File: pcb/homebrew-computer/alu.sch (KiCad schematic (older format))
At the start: 4 parts, among them U4 XC9572XL-10VQG44C

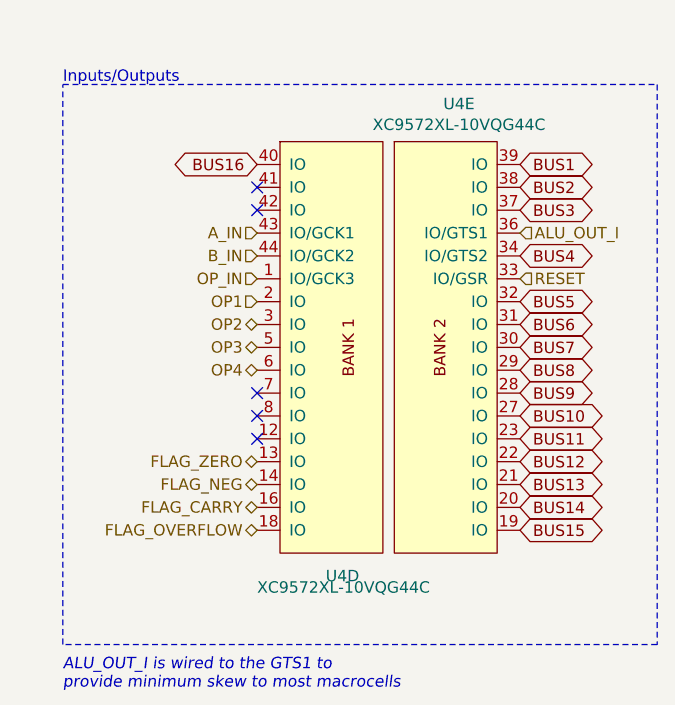
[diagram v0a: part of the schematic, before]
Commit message: Keep working on the layout
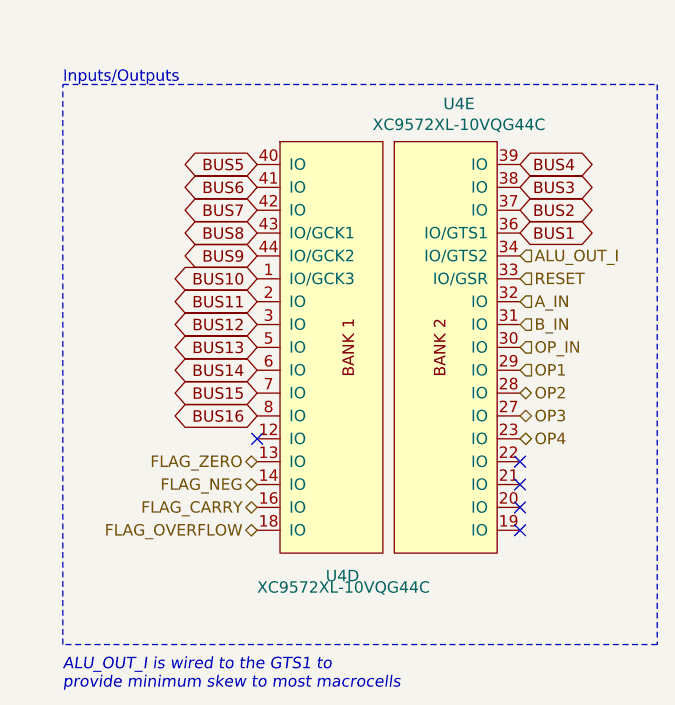
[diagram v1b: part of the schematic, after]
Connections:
- net ALU_OUT_I: now also U4.34 (IO/GTS2); no longer U4.36 (IO/GTS1)
- net A_IN: now also U4.32 (IO); no longer U4.43 (IO/GCK1)
- net BUS1: now also U4.36 (IO/GTS1); no longer U4.39 (IO)
- net BUS10: now also U4.1 (IO/GCK3); no longer U4.27 (IO)
- net BUS11: now also U4.2 (IO); no longer U4.23 (IO)
- net BUS12: now also U4.3 (IO); no longer U4.22 (IO)
- net BUS13: now also U4.5 (IO); no longer U4.21 (IO)
- net BUS14: now also U4.6 (IO); no longer U4.20 (IO)
- net BUS15: now also U4.7 (IO); no longer U4.19 (IO)
- net BUS16: now also U4.8 (IO); no longer U4.40 (IO)
- net BUS2: now also U4.37 (IO); no longer U4.38 (IO)
- net BUS3: now also U4.38 (IO); no longer U4.37 (IO)
- net BUS4: now also U4.39 (IO); no longer U4.34 (IO/GTS2)
- net BUS5: now also U4.40 (IO); no longer U4.32 (IO)
- net BUS6: now also U4.41 (IO); no longer U4.31 (IO)
- net BUS7: now also U4.42 (IO); no longer U4.30 (IO)
- net BUS8: now also U4.43 (IO/GCK1); no longer U4.29 (IO)
- net BUS9: now also U4.44 (IO/GCK2); no longer U4.28 (IO)
- net B_IN: now also U4.31 (IO); no longer U4.44 (IO/GCK2)
- net OP1: now also U4.29 (IO); no longer U4.2 (IO)
- net OP2: now also U4.28 (IO); no longer U4.3 (IO)
- net OP3: now also U4.27 (IO); no longer U4.5 (IO)
- net OP4: now also U4.23 (IO); no longer U4.6 (IO)
- net OP_IN: now also U4.30 (IO); no longer U4.1 (IO/GCK3)
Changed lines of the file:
@@
 Text Notes 1450 3200 0    50   ~ 0
 JTAG
-Text HLabel 5350 1850 0    50   Input ~ 0
+Text HLabel 6500 2150 2    50   Input ~ 0
 OP1
-Text HLabel 5350 1950 0    50   3State ~ 0
+Text HLabel 6500 2250 2    50   3State ~ 0
 OP2
-Text HLabel 5350 2050 0    50   3State ~ 0
+Text HLabel 6500 2350 2    50   3State ~ 0
 OP3
-Text HLabel 5350 2150 0    50   3State ~ 0
+Text HLabel 6500 2450 2    50   3State ~ 0
 OP4
-Text HLabel 5350 2550 0    50   3State ~ 0
-FLAG_ZERO
-Text HLabel 5350 2650 0    50   3State ~ 0
-FLAG_NEG
-Text HLabel 5350 2750 0    50   3State ~ 0
-FLAG_CARRY
-Text HLabel 5350 2850 0    50   3State ~ 0
-FLAG_OVERFLOW
-NoConn ~ 5350 1350
-NoConn ~ 5350 1450
-NoConn ~ 5350 2250
-NoConn ~ 5350 2450
 Wire Notes Line
 	4500 900  7100 900
@@
 Text Notes 4500 900  0    50   ~ 0
 Inputs/Outputs
-Text HLabel 6500 1550 2    50   Input ~ 0
+Text HLabel 6500 1650 2    50   Input ~ 0
 ALU_OUT_I
-Text HLabel 5350 1550 0    50   Input ~ 0
+Text HLabel 6500 1850 2    50   Input ~ 0
 A_IN
-Text HLabel 5350 1650 0    50   Input ~ 0
+Text HLabel 6500 1950 2    50   Input ~ 0
 B_IN
-Text HLabel 5350 1750 0    50   Input ~ 0
+Text HLabel 6500 2050 2    50   Input ~ 0
 OP_IN
 $Comp
@@
 Text HLabel 6500 1750 2    50   Input ~ 0
 RESET
-NoConn ~ 5350 2350
 Text Notes 4500 3550 0    50   Italic 0
 ALU_OUT_I is wired to the GTS1 to\nprovide minimum skew to most macrocells
 Text Notes 4500 3800 0    50   Italic 0
 RESET is wired to GSR to\nprovide minimum skew to most macrocells
+Text GLabel 5350 2350 0    50   3State ~ 0
+BUS16
+Text GLabel 5350 2250 0    50   3State ~ 0
+BUS15
+Text GLabel 5350 2150 0    50   3State ~ 0
+BUS14
+Text GLabel 5350 2050 0    50   3State ~ 0
+BUS13
+Text GLabel 5350 1950 0    50   3State ~ 0
+BUS12
+Text GLabel 5350 1850 0    50   3State ~ 0
+BUS11
+Text GLabel 5350 1750 0    50   3State ~ 0
+BUS10
+Text GLabel 5350 1650 0    50   3State ~ 0
+BUS9
+Text GLabel 5350 1550 0    50   3State ~ 0
+BUS8
+Text GLabel 5350 1450 0    50   3State ~ 0
+BUS7
+Text GLabel 5350 1350 0    50   3State ~ 0
+BUS6
 Text GLabel 5350 1250 0    50   3State ~ 0
-BUS16
-Text GLabel 6500 2850 2    50   3State ~ 0
-BUS15
-Text GLabel 6500 2750 2    50   3State ~ 0
-BUS14
-Text GLabel 6500 2650 2    50   3State ~ 0
-BUS13
-Text GLabel 6500 2550 2    50   3State ~ 0
-BUS12
-Text GLabel 6500 2450 2    50   3State ~ 0
-BUS11
-Text GLabel 6500 2350 2    50   3State ~ 0
-BUS10
-Text GLabel 6500 2250 2    50   3State ~ 0
-BUS9
-Text GLabel 6500 2150 2    50   3State ~ 0
-BUS8
-Text GLabel 6500 2050 2    50   3State ~ 0
-BUS7
-Text GLabel 6500 1950 2    50   3State ~ 0
-BUS6
-Text GLabel 6500 1850 2    50   3State ~ 0
 BUS5
-Text GLabel 6500 1650 2    50   3State ~ 0
+Text GLabel 6500 1250 2    50   3State ~ 0
 BUS4
+Text GLabel 6500 1350 2    50   3State ~ 0
+BUS3
 Text GLabel 6500 1450 2    50   3State ~ 0
-BUS3
-Text GLabel 6500 1350 2    50   3State ~ 0
 BUS2
-Text GLabel 6500 1250 2    50   3State ~ 0
+Text GLabel 6500 1550 2    50   3State ~ 0
 BUS1
 Wire Wire Line
@@
 Wire Wire Line
 	2050 1800 2400 1800
+NoConn ~ 6500 2850
+NoConn ~ 6500 2750
+NoConn ~ 6500 2650
+NoConn ~ 6500 2550
+NoConn ~ 5350 2450
+Text HLabel 5350 2850 0    50   3State ~ 0
+FLAG_OVERFLOW
+Text HLabel 5350 2750 0    50   3State ~ 0
+FLAG_CARRY
+Text HLabel 5350 2650 0    50   3State ~ 0
+FLAG_NEG
+Text HLabel 5350 2550 0    50   3State ~ 0
+FLAG_ZERO
 $EndSCHEMATC
